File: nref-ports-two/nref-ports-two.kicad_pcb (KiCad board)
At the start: 4 copper layers, 87.5 x 40.2 mm, 117 parts, among them J1 USB_C_Receptacle, J2 USB_C_Receptacle, J3 USB3_A, J4 HD0919MSMTTR, J5 Conn_01x20, J6 Conn_01x12_Pin, J7 Conn_01x04, U1 TUSB8041, U10 TPD4E02B04DQA, U11 TPD12S521, U12 LM2830XQMFE/NOPB, U13 LM2830XQMFE/NOPB, U2 HD3SS3220IRNHT, U3 TPD4E02B04DQA, U4 TPD4E02B04DQA, U5 TPD4E02B04DQA, U6 TPD4E02B04DQA, U7 TPD4E02B04DQA, U8 TPD4E02B04DQA, U9 TPD4E02B04DQA, Y1 24MHz

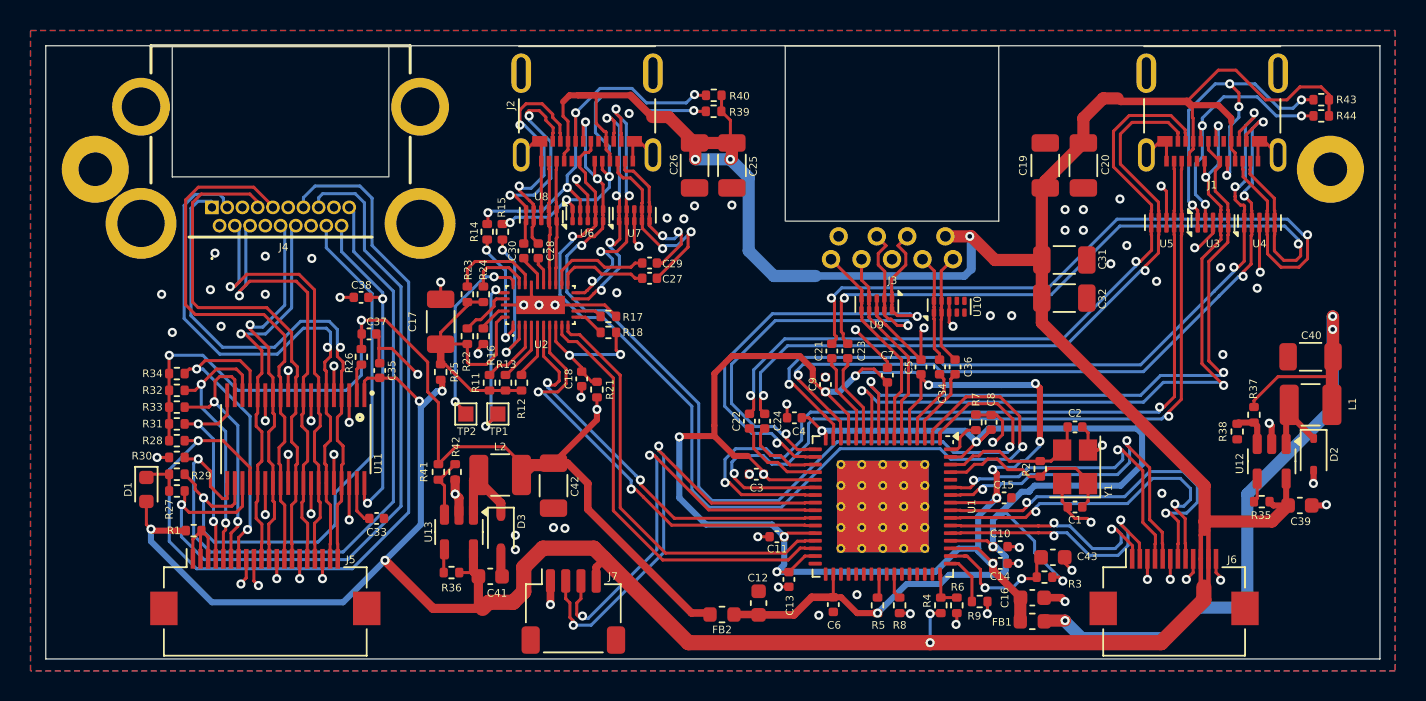
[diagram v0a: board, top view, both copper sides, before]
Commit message: add latest PCB updates
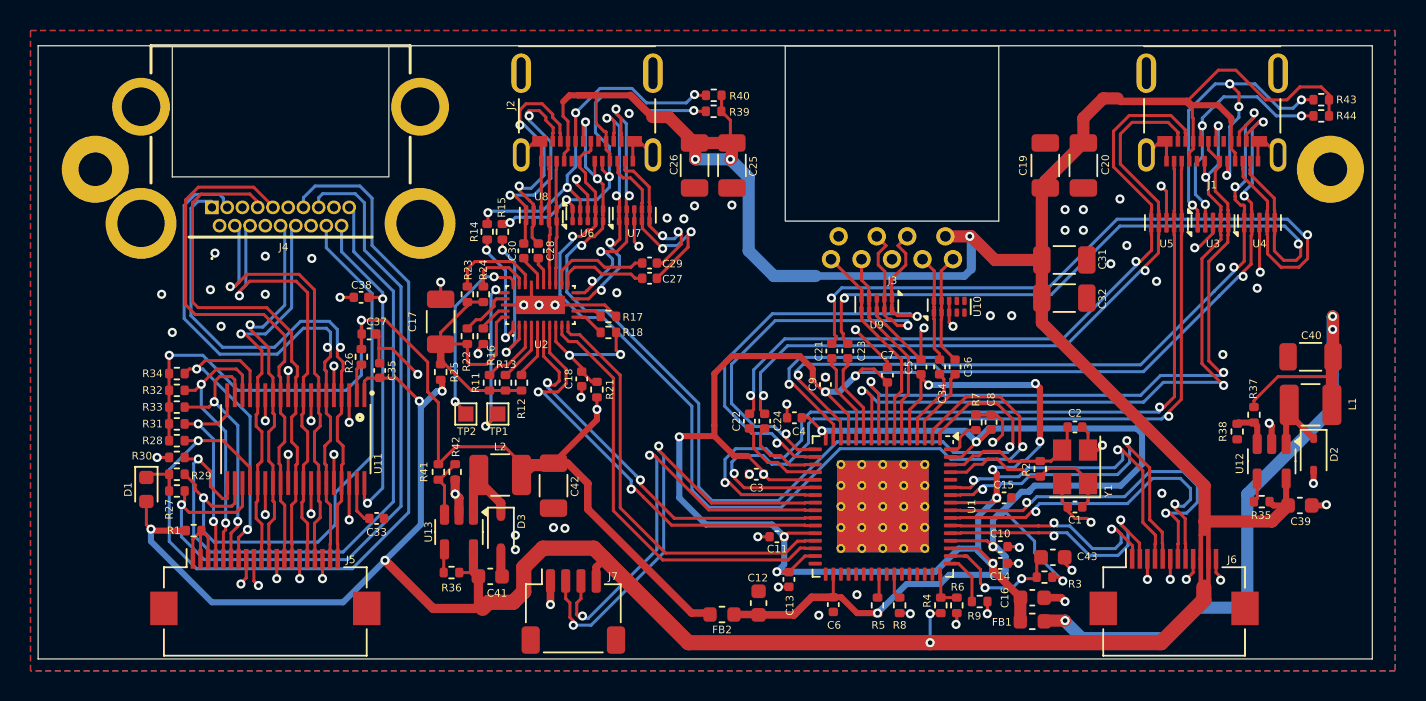
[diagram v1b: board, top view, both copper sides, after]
